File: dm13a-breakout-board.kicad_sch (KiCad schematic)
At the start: 6 parts, among them J1 Conn_01x16, J2 Conn_01x02, J3 Conn_01x05, U1 DM13A

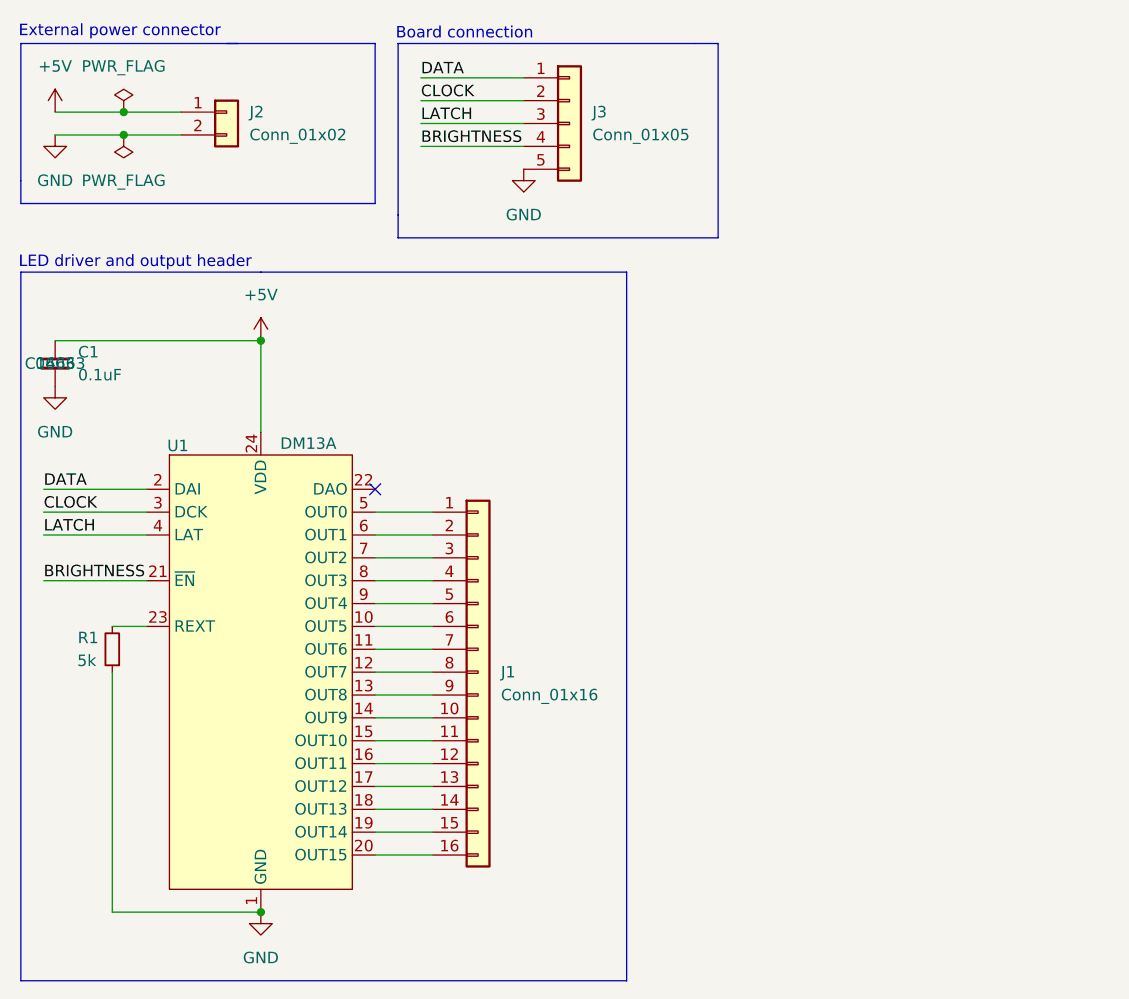
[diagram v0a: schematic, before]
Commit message: Try the whole thing
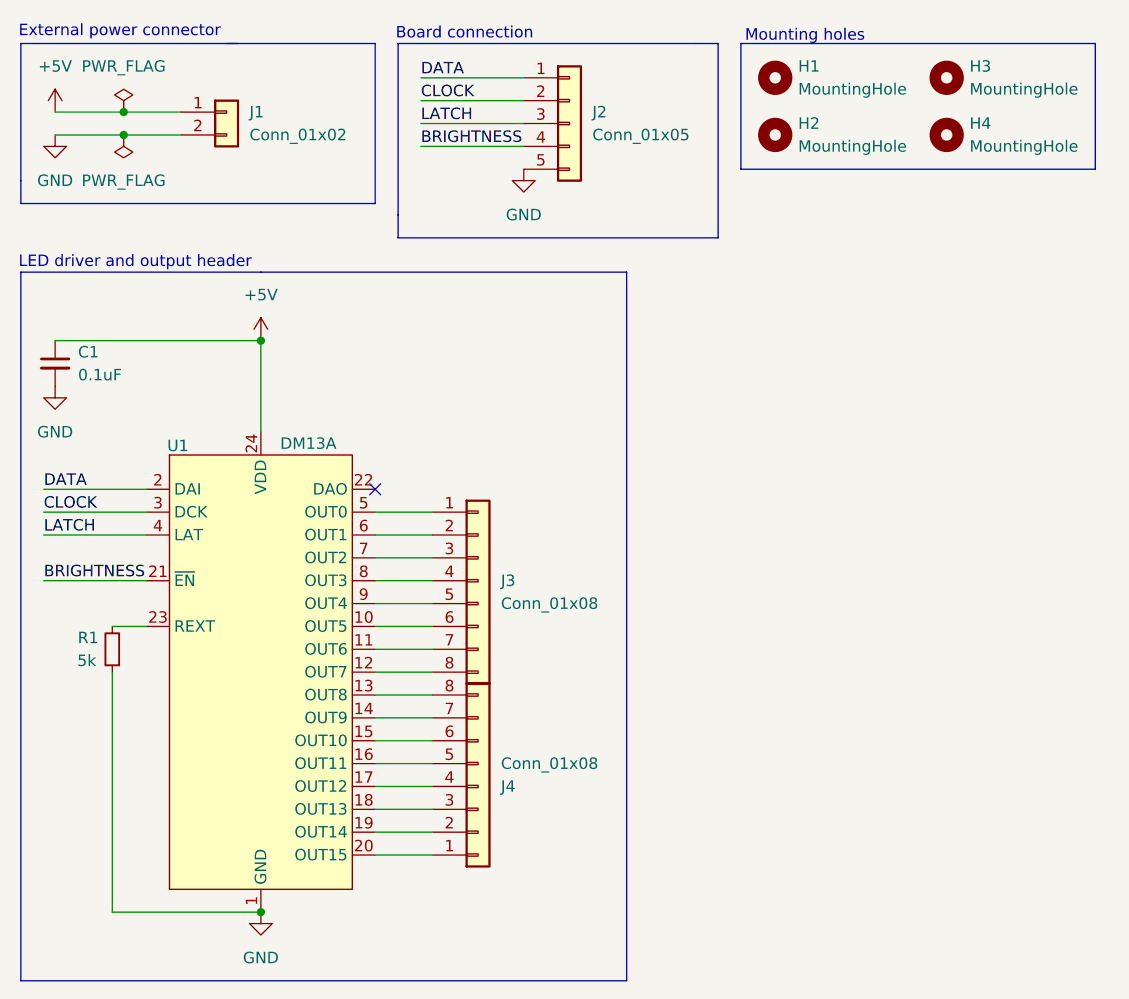
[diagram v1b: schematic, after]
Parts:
- removed J1: Conn_01x16, symbol Connector_Generic:Conn_01x16
- added H1, H2, H3, H4: MountingHole, MountingHole:MountingHole_3.2mm_M3, symbol Mechanical:MountingHole
- added J3, J4: Conn_01x08, Connector_PinHeader_2.54mm:PinHeader_1x08_P2.54mm_Vertical, symbol Connector_Generic:Conn_01x08
- J1: renamed from J2; footprint (none) -> Connector_PinHeader_2.54mm:PinHeader_1x02_P2.54mm_Vertical
- J2: renamed from J3; footprint (none) -> Connector_PinHeader_2.54mm:PinHeader_1x05_P2.54mm_Vertical
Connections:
- net at U1.5 (OUT0): now also J3.1 (Pin_1)
- net at U1.14 (OUT9): now also J4.7 (Pin_7)
- net at U1.15 (OUT10): now also J4.6 (Pin_6)
- net at U1.16 (OUT11): now also J4.5 (Pin_5)
- net at U1.17 (OUT12): now also J4.4 (Pin_4)
- net at U1.18 (OUT13): now also J4.3 (Pin_3)
- net at U1.19 (OUT14): now also J4.2 (Pin_2)
- net at U1.20 (OUT15): now also J4.1 (Pin_1)
- net at U1.6 (OUT1): now also J3.2 (Pin_2)
- net at U1.7 (OUT2): now also J3.3 (Pin_3)
- net at U1.8 (OUT3): now also J3.4 (Pin_4)
- net at U1.9 (OUT4): now also J3.5 (Pin_5)
- net at U1.10 (OUT5): now also J3.6 (Pin_6)
- net at U1.11 (OUT6): now also J3.7 (Pin_7)
- net at U1.12 (OUT7): now also J3.8 (Pin_8)
- net at U1.13 (OUT8): now also J4.8 (Pin_8)
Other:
- note added: "Mounting holes"
